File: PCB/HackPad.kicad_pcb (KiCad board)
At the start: 2 copper layers, 83.4 x 121.3 mm, 34 parts, among them SW1 RotaryEncoder_Switch_MP, SW10 SW_Push_45deg, SW11 SW_Push_45deg, SW12 SW_Push_45deg, SW13 SW_Push_45deg, SW14 SW_Push_45deg, SW15 SW_Push_45deg, SW16 SW_Push_45deg, SW17 SW_Push_45deg, SW2 SW_Push_45deg, SW3 SW_Push_45deg, SW4 SW_Push_45deg, SW5 SW_Push_45deg, SW6 SW_Push_45deg, SW7 SW_Push_45deg, SW8 SW_Push_45deg, SW9 SW_Push_45deg, U1 XIAO-RP2040-DIP

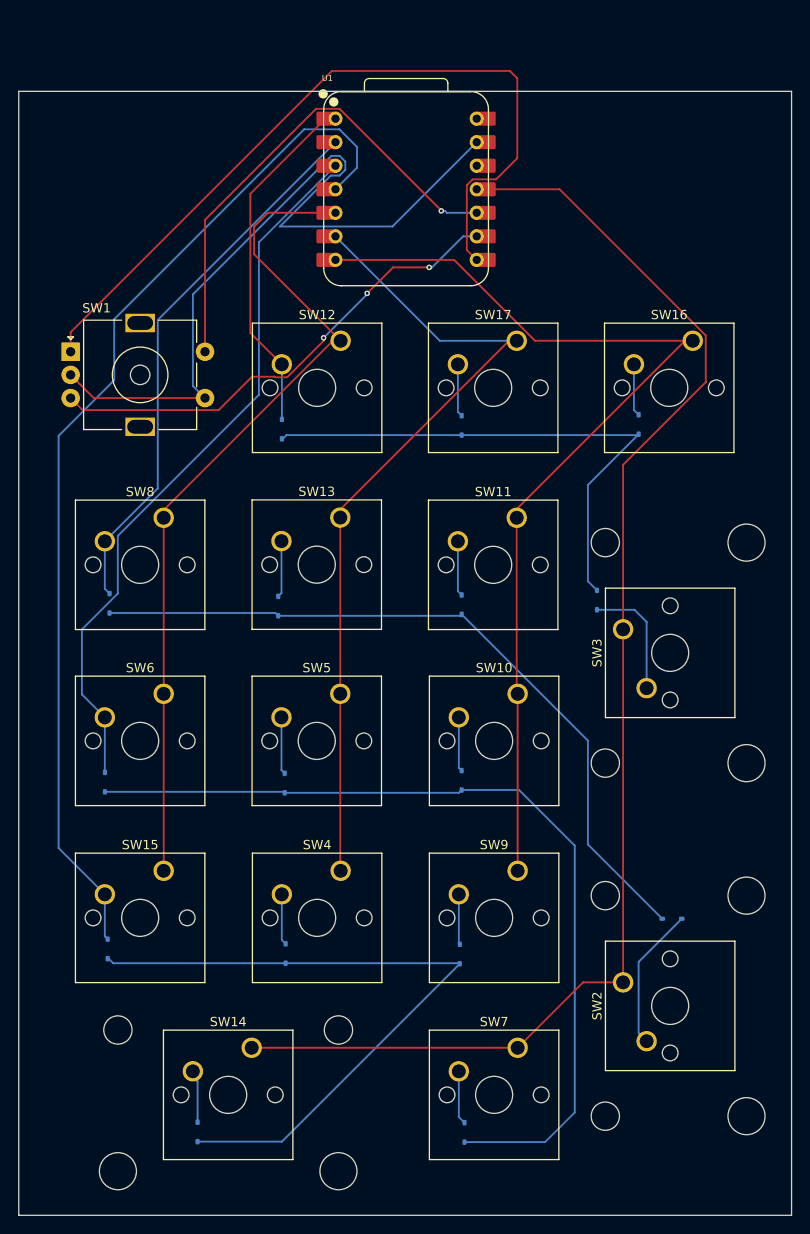
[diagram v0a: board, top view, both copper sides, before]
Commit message: Add files via upload
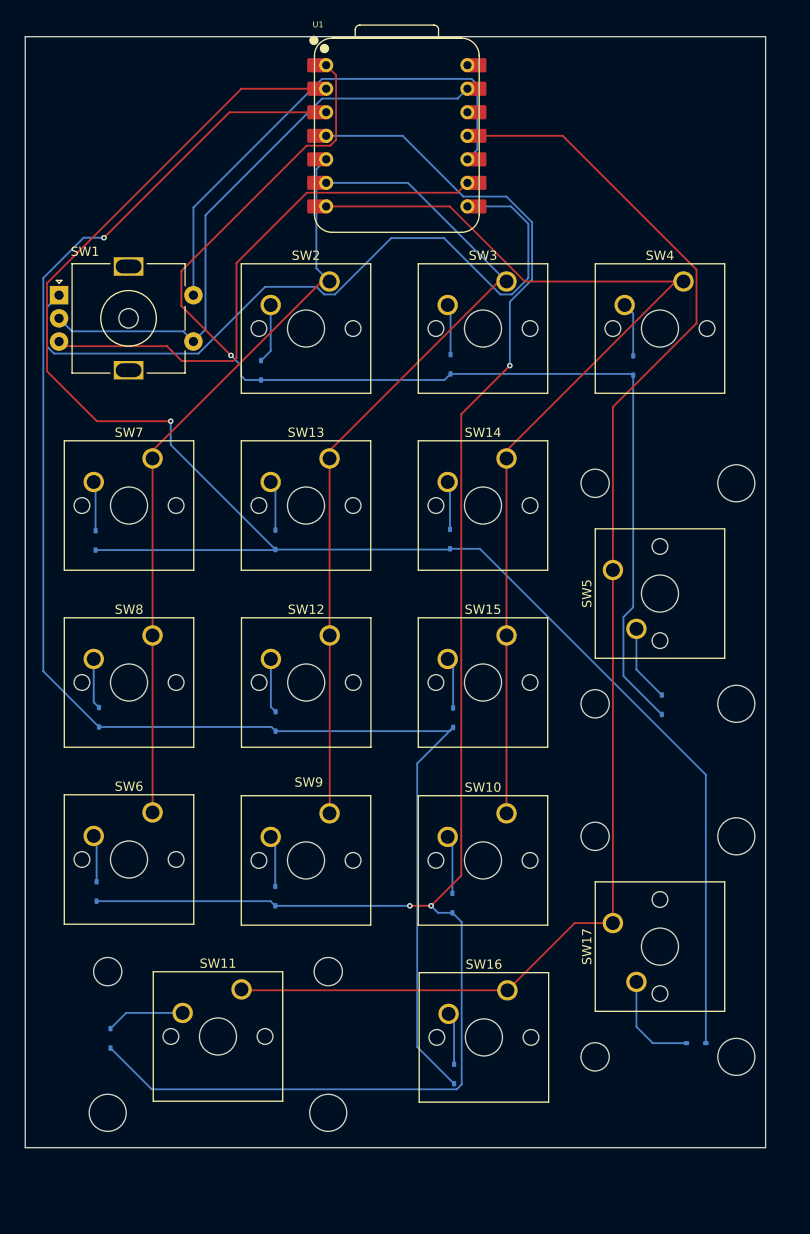
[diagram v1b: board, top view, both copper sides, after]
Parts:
- SW11, SW17, SW5: footprint Button_Switch_Keyboard:SW_Cherry_MX_1.00u_PCB -> Button_Switch_Keyboard:SW_Cherry_MX_2.00u_PCB
- SW14, SW2, SW3: footprint Button_Switch_Keyboard:SW_Cherry_MX_2.00u_PCB -> Button_Switch_Keyboard:SW_Cherry_MX_1.00u_PCB
- moved D10 87.4 mm to (51.8, 169.1)
- moved D1 82.5 mm to (68.0, 97.0)
- moved SW2 82.0 mm to (75.4, 87.4), turned to 0 degrees
- moved SW7 74.8 mm to (56.3, 106.5)
- moved SW4 73.6 mm to (113.6, 87.4)
- moved SW16 72.9 mm to (94.6, 163.9)
- moved SW14 69.3 mm to (94.5, 106.5)
- moved D6 65.6 mm to (50.6, 134.4), turned to 90 degrees
- moved SW17 63.7 mm to (106.0, 156.7), turned to 90 degrees
- moved SW11 58.9 mm to (65.9, 163.8)
- moved D9 49.1 mm to (88.7, 154.5)
- moved D15 49.1 mm to (88.9, 172.9)
- moved D5 49.1 mm to (50.2, 115.4)
- moved SW15 44.9 mm to (94.5, 125.6)
- moved D14 44.8 mm to (88.8, 134.5)
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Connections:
- D1 pad 1: ROW3 -> ROW0
- D10 pad 1: ROW0 -> ROW3
- D10 pad 2: (no net) -> Net-(D10-A)
- D11 pad 1: ROW1 -> ROW2
- D11 pad 2: (no net) -> Net-(D11-A)
- D12 pad 2: (no net) -> Net-(D12-A)
- D13 pad 1: ROW0 -> ROW1
- D13 pad 2: (no net) -> Net-(D13-A)
- D14 pad 2: (no net) -> Net-(D14-A)
- D15 pad 2: (no net) -> Net-(D15-A)
- D16 pad 1: ROW2 -> ROW1
- D16 pad 2: (no net) -> Net-(D16-A)
- D2 pad 1: (no net) -> ROW0
- D2 pad 2: (no net) -> Net-(D2-A)
- D3 pad 2: (no net) -> Net-(D3-A)
- D4 pad 1: ROW2 -> ROW0
- D5 pad 1: ROW3 -> ROW1
- D5 pad 2: (no net) -> Net-(D5-A)
- D6 pad 1: ROW1 -> ROW2
- D6 pad 2: (no net) -> Net-(D6-A)
- D7 pad 2: (no net) -> Net-(D7-A)
- D9 pad 1: ROW1 -> ROW3
- D9 pad 2: (no net) -> Net-(D9-A)
- SW1 pad S2: (no net) -> Net-(U1-GPIO4/MISO)
- SW10 pad 2: (no net) -> Net-(D9-A)
- SW11 pad 1: COL2 -> COL3
- SW11 pad 2: (no net) -> Net-(D10-A)
- SW12 pad 1: COL0 -> COL1
- SW12 pad 2: (no net) -> Net-(D11-A)
- SW13 pad 2: (no net) -> Net-(D12-A)
- SW14 pad 1: COL3 -> COL2
- SW14 pad 2: Net-(D1-A) -> Net-(D13-A)
- SW15 pad 1: COL0 -> COL2
- SW15 pad 2: (no net) -> Net-(D14-A)
- SW16 pad 1: COL2 -> COL3
- SW16 pad 2: (no net) -> Net-(D15-A)
- SW17 pad 1: COL1 -> COL3
- SW17 pad 2: (no net) -> Net-(D16-A)
- SW2 pad 1: COL3 -> COL0
- SW2 pad 2: (no net) -> Net-(D1-A)
- SW3 pad 1: COL3 -> COL1
- SW3 pad 2: (no net) -> Net-(D2-A)
- SW4 pad 1: COL1 -> COL2
- SW4 pad 2: (no net) -> Net-(D3-A)
- SW5 pad 1: COL1 -> COL3
- SW6 pad 2: (no net) -> Net-(D7-A)
- SW7 pad 1: COL3 -> COL0
- SW7 pad 2: (no net) -> Net-(D5-A)
- SW8 pad 2: (no net) -> Net-(D6-A)
- SW9 pad 1: COL2 -> COL1
- U1 pad 10: unconnected-(U1-GPIO4/MISO-Pad10) -> Net-(U1-GPIO4/MISO)
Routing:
- net (no net): track 59.0 -> 0.00 mm, vias 1 -> 0
- net Net-(U1-GPIO4/MISO): track 0.00 -> 54.6 mm
- net GND: track 85.6 -> 63.6 mm
- net ROW1: track 166.8 -> 187.4 mm, vias 0 -> 1
- net Net-(D16-A): track 0.00 -> 11.0 mm
- net ROW2: track 179.1 -> 169.2 mm, vias 0 -> 1
- net COL0: track 91.2 -> 81.5 mm
- net ROW3: track 192.6 -> 202.2 mm, vias 0 -> 3
- net Net-(D10-A): track 0.00 -> 8.49 mm
- net Net-(U1-GPIO2/SCK): track 52.4 -> 58.9 mm, vias 3 -> 0
- net Net-(D9-A): track 0.00 -> 6.30 mm
- net Net-(D11-A): track 0.00 -> 5.90 mm
- net Net-(D3-A): track 0.00 -> 5.86 mm
- net ROW0: track 120.9 -> 126.6 mm, vias 0 -> 1
- net Net-(D15-A): track 0.00 -> 5.68 mm
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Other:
- board size 83.4 x 121.3 mm -> 79.9 x 119.9 mm
